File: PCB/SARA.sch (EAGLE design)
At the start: 46 parts, among them J1 1935161, J2 PJ-002AH, U1 MAX9110EKA+T, U2 MAX9110EKA+T, U3 MAX9111EKA+T, U4 MAX9111EKA+T, U5 R-78B3.3-2.0, U6 R-78B3.3-2.0

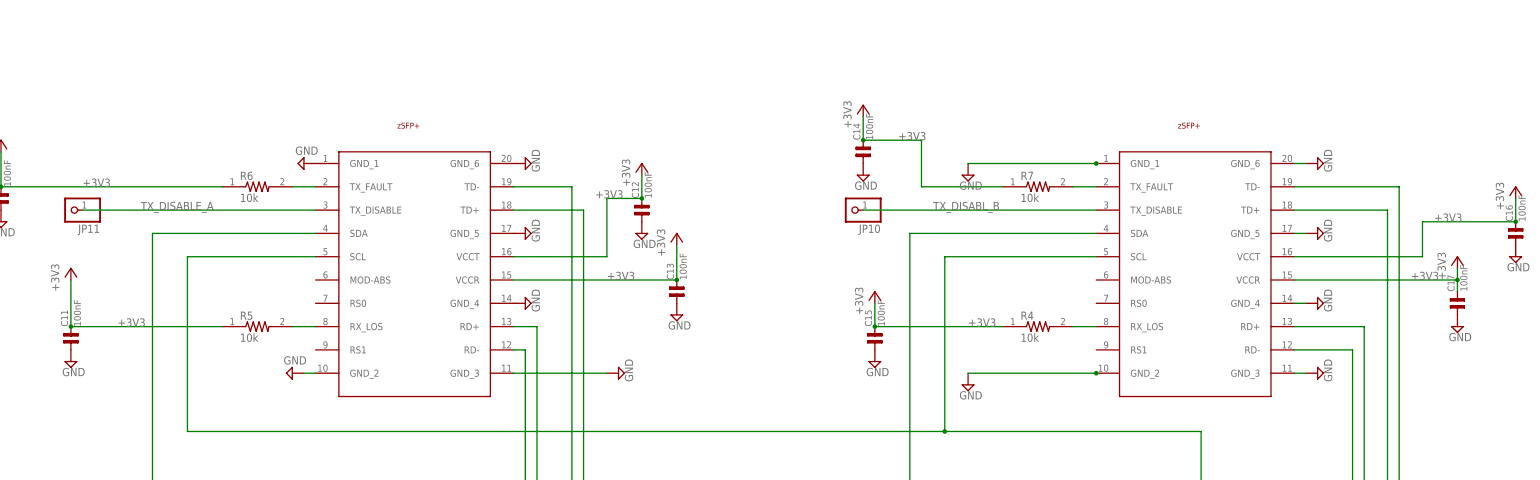
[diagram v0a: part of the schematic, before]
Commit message: Added Tim's PCB v2 files
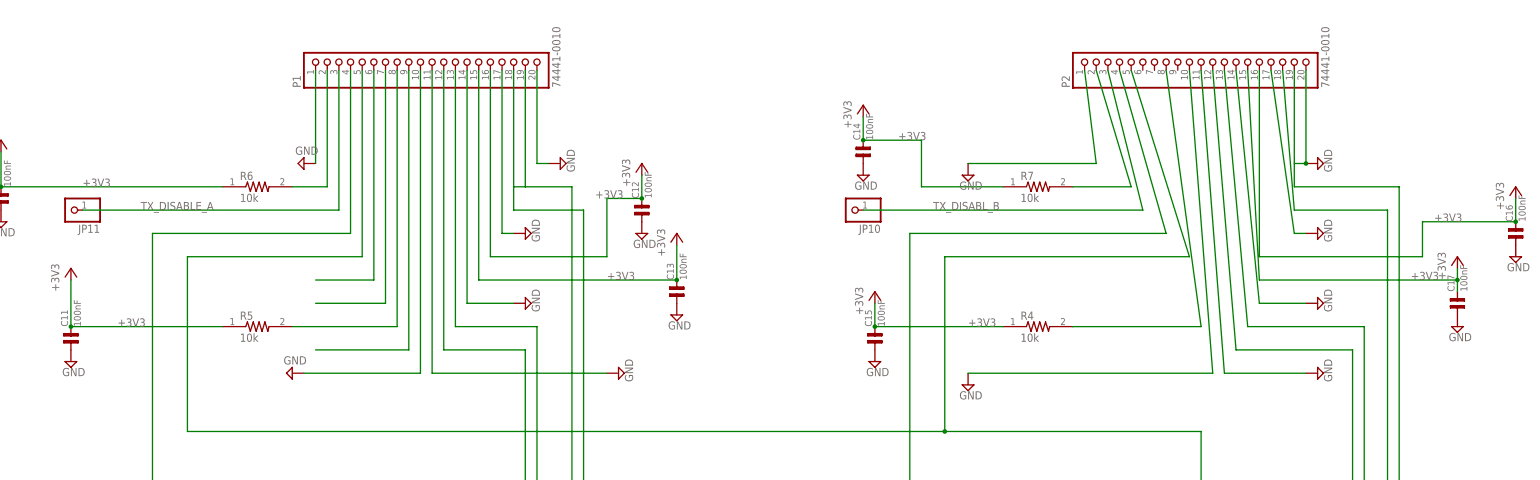
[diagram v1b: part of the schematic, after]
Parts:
- removed SFP_DOWNSTREAM, SFP_UPSTREAM: ZSFP+, zSFP+:ZSFP+
- added P1, P2: 74441-0010, 74441-0010:74441-0010
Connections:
- new net N$3: P1.6
- new net N$5: P1.7
- new net N$6: P1.9
- net +3V3: now also P1.15, P1.16, P2.15, P2.16; no longer SFP_DOWNSTREAM.VCCR, SFP_DOWNSTREAM.VCCT, SFP_UPSTREAM.VCCR, SFP_UPSTREAM.VCCT
- net GND: now also P1.1, P1.10, P1.11, P1.14, P1.17, P1.20, P2.1, P2.11, P2.14, P2.17, P2.20; no longer SFP_DOWNSTREAM.GND_1, SFP_DOWNSTREAM.GND_2, SFP_DOWNSTREAM.GND_3, SFP_DOWNSTREAM.GND_4, SFP_DOWNSTREAM.GND_5, SFP_DOWNSTREAM.GND_6, SFP_UPSTREAM.GND_1, SFP_UPSTREAM.GND_3, SFP_UPSTREAM.GND_4, SFP_UPSTREAM.GND_5, SFP_UPSTREAM.GND_6
- net I2C_SCL: now also P1.5, P2.5; no longer SFP_DOWNSTREAM.SCL, SFP_UPSTREAM.SCL
- net I2C_SDA: now also P1.4, P2.4; no longer SFP_DOWNSTREAM.SDA, SFP_UPSTREAM.SDA
- net N$1: now also P2.8; no longer SFP_UPSTREAM.RX_LOS
- net N$19: now also P1.8; no longer SFP_DOWNSTREAM.RX_LOS
- net N$20: now also P1.2; no longer SFP_DOWNSTREAM.TX_FAULT
- net N$21: now also P2.2; no longer SFP_UPSTREAM.TX_FAULT
- net N$7: now also P2.10; no longer SFP_UPSTREAM.GND_2
- net RXD_N: now also P2.12; no longer SFP_UPSTREAM.RD-
- net RXD_P: now also P2.13; no longer SFP_UPSTREAM.RD+
- net RXL_N: now also P1.12; no longer SFP_DOWNSTREAM.RD-
- net RXL_P: now also P1.13; no longer SFP_DOWNSTREAM.RD+
- net TXD_N: now also P2.19; no longer SFP_UPSTREAM.TD-
- net TXD_P: now also P2.18; no longer SFP_UPSTREAM.TD+
- net TXL_N: now also P1.19; no longer SFP_DOWNSTREAM.TD-
- net TXL_P: now also P1.18; no longer SFP_DOWNSTREAM.TD+
- net TX_DISABLE_A: now also P1.3; no longer SFP_DOWNSTREAM.TX_DISABLE
- net TX_DISABL_B: now also P2.3; no longer SFP_UPSTREAM.TX_DISABLE
